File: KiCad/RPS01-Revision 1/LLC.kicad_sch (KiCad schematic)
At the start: 12 parts, among them Q1 BSS138, Q2 BSS138

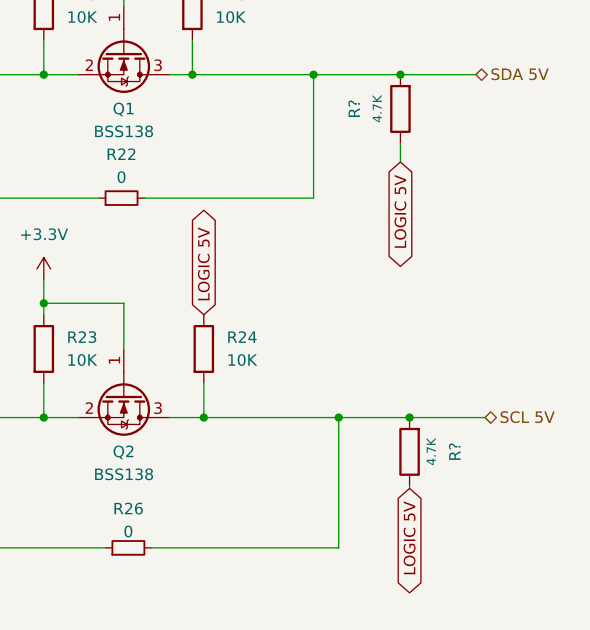
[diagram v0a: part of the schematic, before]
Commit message: update
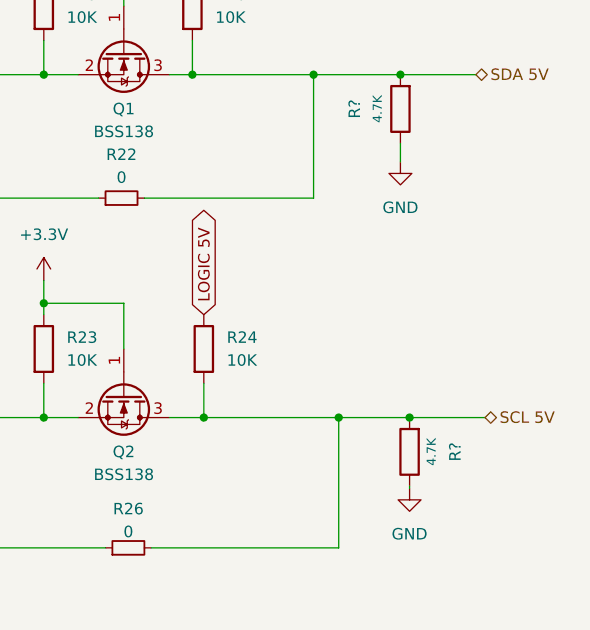
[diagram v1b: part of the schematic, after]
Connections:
- net LOGIC 5V: no longer R?.1, R?.1
- new net GND: R?.1, R?.1
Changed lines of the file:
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@@
-    )
-  )
-  (global_label "LOGIC 5V" (shape bidirectional) (at 186.944 107.4928 270) (fields_autoplaced)
-    (effects (font (size 1.27 1.27)) (justify right))
-    (property "Intersheetrefs" "${INTERSHEET_REFS}" (at 186.944 120.279 90)
-      (effects (font (size 1.27 1.27)) (justify right) hide)
-    )
-  )
-  (global_label "LOGIC 5V" (shape bidirectional) (at 187.96 143.764 270) (fields_autoplaced)
-    (effects (font (size 1.27 1.27)) (justify right))
-    (property "Intersheetrefs" "${INTERSHEET_REFS}" (at 187.96 156.5502 90)
-      (effects (font (size 1.27 1.27)) (justify right) hide)
     )
   )
@@
     )
   )
+  (symbol (lib_id "power:GND") (at 187.96 143.764 0) (unit 1)
+    (in_bom yes) (on_board yes) (dnp no) (fields_autoplaced)
+    (property "Reference" "#PWR?" (at 187.96 150.114 0)
+      (effects (font (size 1.27 1.27)) hide)
+    )
+    (property "Value" "GND" (at 187.96 148.844 0)
+      (effects (font (size 1.27 1.27)))
+    )
+    (property "Footprint" "" (at 187.96 143.764 0)
+      (effects (font (size 1.27 1.27)) hide)
+    )
+    (property "Datasheet" "" (at 187.96 143.764 0)
+      (effects (font (size 1.27 1.27)) hide)
+    )
+    (pin "1")
+    (instances
+      (project "MCU2"
+        (path "/049009a7-95d1-4ccf-a10c-7859cfd6b188"
+          (reference "#PWR?") (unit 1)
+        )
+      )
+      (project "rps01"
+        (path "/14930f15-c0a0-4b55-93e6-b112548415f6/a2e49fe6-126d-427d-b045-54fb7f662aa7"
+          (reference "#PWR?") (unit 1)
+        )
+        (path "/14930f15-c0a0-4b55-93e6-b112548415f6/c06f7478-c874-4c9c-9b0f-f3b722914738"
+          (reference "#PWR067") (unit 1)
+        )
+      )
+    )
+  )
   (symbol (lib_id "Device:R_Small") (at 156.718 150.368 90) (unit 1)
     (in_bom yes) (on_board yes) (dnp no) (fields_autoplaced)
@@
         )
       )
+    )
+  )
+  (symbol (lib_id "power:GND") (at 186.944 107.4928 0) (unit 1)
+    (in_bom yes) (on_board yes) (dnp no) (fields_autoplaced)
+    (property "Reference" "#PWR?" (at 186.944 113.8428 0)
+      (effects (font (size 1.27 1.27)) hide)
+    )
+    (property "Value" "GND" (at 186.944 112.5728 0)
+      (effects (font (size 1.27 1.27)))
+    )
+    (property "Footprint" "" (at 186.944 107.4928 0)
+      (effects (font (size 1.27 1.27)) hide)
+    )
+    (property "Datasheet" "" (at 186.944 107.4928 0)
+      (effects (font (size 1.27 1.27)) hide)
+    )
+    (pin "1")
+    (instances
+      (project "MCU2"
+        (path "/049009a7-95d1-4ccf-a10c-7859cfd6b188"
+          (reference "#PWR?") (unit 1)
+        )
+      )
+      (project "rps01"
+        (path "/14930f15-c0a0-4b55-93e6-b112548415f6/a2e49fe6-126d-427d-b045-54fb7f662aa7"
+          (reference "#PWR?") (unit 1)
+        )
+        (path "/14930f15-c0a0-4b55-93e6-b112548415f6/c06f7478-c874-4c9c-9b0f-f3b722914738"
+          (reference "#PWR065") (unit 1)
+        )
+      )

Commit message: update
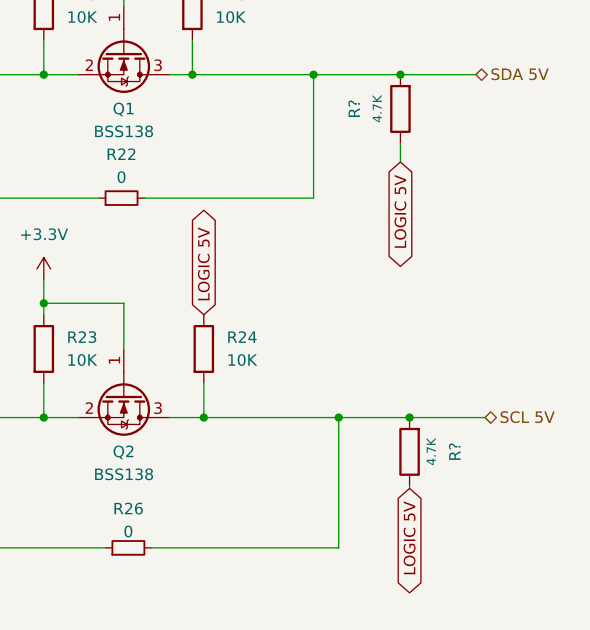
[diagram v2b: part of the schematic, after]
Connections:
- net GND is gone; now on net LOGIC 5V: R?.1, R?.1
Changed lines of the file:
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@@
+    )
+  )
+  (global_label "LOGIC 5V" (shape bidirectional) (at 186.944 107.4928 270) (fields_autoplaced)
+    (effects (font (size 1.27 1.27)) (justify right))
+    (property "Intersheetrefs" "${INTERSHEET_REFS}" (at 186.944 120.279 90)
+      (effects (font (size 1.27 1.27)) (justify right) hide)
+    )
+  )
+  (global_label "LOGIC 5V" (shape bidirectional) (at 187.96 143.764 270) (fields_autoplaced)
+    (effects (font (size 1.27 1.27)) (justify right))
+    (property "Intersheetrefs" "${INTERSHEET_REFS}" (at 187.96 156.5502 90)
+      (effects (font (size 1.27 1.27)) (justify right) hide)
     )
   )
@@
     )
   )
-  (symbol (lib_id "power:GND") (at 187.96 143.764 0) (unit 1)
-    (in_bom yes) (on_board yes) (dnp no) (fields_autoplaced)
-    (property "Reference" "#PWR?" (at 187.96 150.114 0)
-      (effects (font (size 1.27 1.27)) hide)
-    )
-    (property "Value" "GND" (at 187.96 148.844 0)
-      (effects (font (size 1.27 1.27)))
-    )
-    (property "Footprint" "" (at 187.96 143.764 0)
-      (effects (font (size 1.27 1.27)) hide)
-    )
-    (property "Datasheet" "" (at 187.96 143.764 0)
-      (effects (font (size 1.27 1.27)) hide)
-    )
-    (pin "1")
-    (instances
-      (project "MCU2"
-        (path "/049009a7-95d1-4ccf-a10c-7859cfd6b188"
-          (reference "#PWR?") (unit 1)
-        )
-      )
-      (project "rps01"
-        (path "/14930f15-c0a0-4b55-93e6-b112548415f6/a2e49fe6-126d-427d-b045-54fb7f662aa7"
-          (reference "#PWR?") (unit 1)
-        )
-        (path "/14930f15-c0a0-4b55-93e6-b112548415f6/c06f7478-c874-4c9c-9b0f-f3b722914738"
-          (reference "#PWR067") (unit 1)
-        )
-      )
-    )
-  )
   (symbol (lib_id "Device:R_Small") (at 156.718 150.368 90) (unit 1)
     (in_bom yes) (on_board yes) (dnp no) (fields_autoplaced)
@@
         )
       )
-    )
-  )
-  (symbol (lib_id "power:GND") (at 186.944 107.4928 0) (unit 1)
-    (in_bom yes) (on_board yes) (dnp no) (fields_autoplaced)
-    (property "Reference" "#PWR?" (at 186.944 113.8428 0)
-      (effects (font (size 1.27 1.27)) hide)
-    )
-    (property "Value" "GND" (at 186.944 112.5728 0)
-      (effects (font (size 1.27 1.27)))
-    )
-    (property "Footprint" "" (at 186.944 107.4928 0)
-      (effects (font (size 1.27 1.27)) hide)
-    )
-    (property "Datasheet" "" (at 186.944 107.4928 0)
-      (effects (font (size 1.27 1.27)) hide)
-    )
-    (pin "1")
-    (instances
-      (project "MCU2"
-        (path "/049009a7-95d1-4ccf-a10c-7859cfd6b188"
-          (reference "#PWR?") (unit 1)
-        )
-      )
-      (project "rps01"
-        (path "/14930f15-c0a0-4b55-93e6-b112548415f6/a2e49fe6-126d-427d-b045-54fb7f662aa7"
-          (reference "#PWR?") (unit 1)
-        )
-        (path "/14930f15-c0a0-4b55-93e6-b112548415f6/c06f7478-c874-4c9c-9b0f-f3b722914738"
-          (reference "#PWR065") (unit 1)
-        )
-      )
